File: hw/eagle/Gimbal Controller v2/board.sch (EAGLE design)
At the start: 3 parts

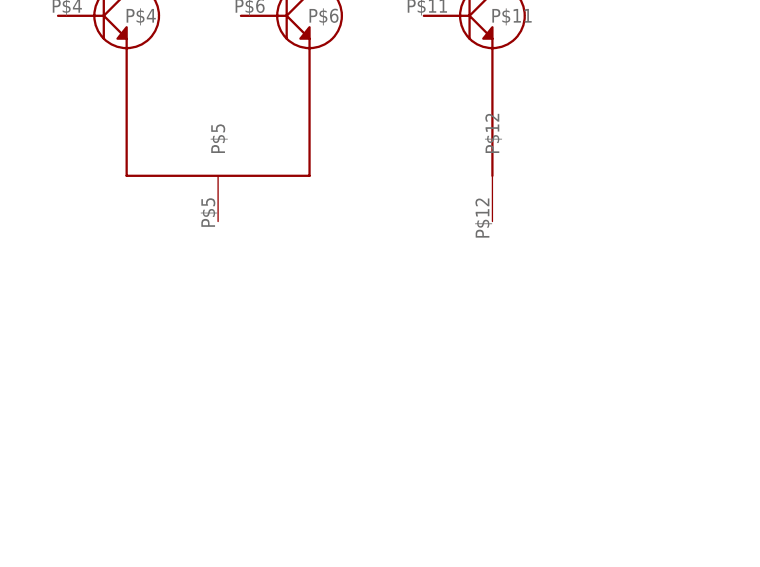
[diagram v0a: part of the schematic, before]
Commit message: gitignore test
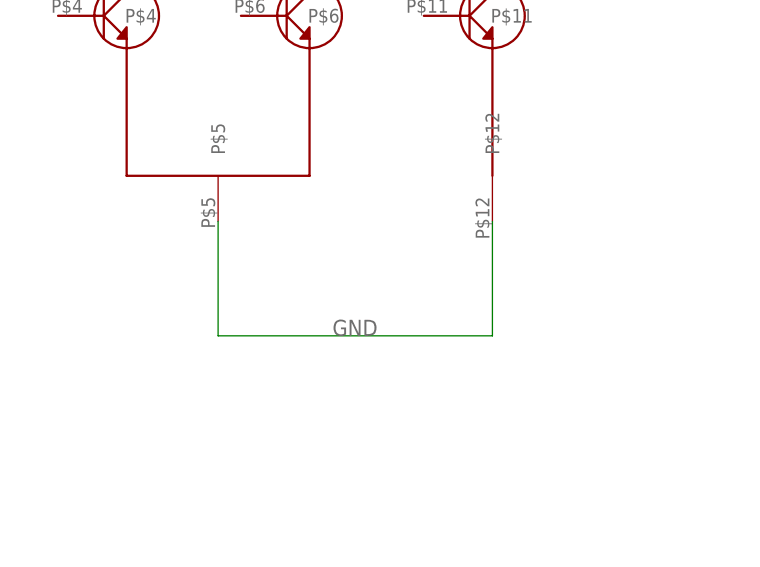
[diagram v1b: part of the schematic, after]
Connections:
- net GND: now also U$2.P$12, U$2.P$5
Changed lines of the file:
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@@
 <label x="-175.26" y="-73.66" size="1.778" layer="95"/>
+</segment>
+<segment>
+<pinref part="U$2" gate="G$1" pin="P$5"/>
+<wire x1="-182.88" y1="147.32" x2="-182.88" y2="134.62" width="0.1524" layer="91"/>
+<pinref part="U$2" gate="G$1" pin="P$12"/>
+<wire x1="-182.88" y1="134.62" x2="-152.4" y2="134.62" width="0.1524" layer="91"/>
+<wire x1="-152.4" y1="134.62" x2="-152.4" y2="147.32" width="0.1524" layer="91"/>
+<label x="-170.18" y="134.62" size="1.778" layer="95"/>
 </segment>
 </net>
